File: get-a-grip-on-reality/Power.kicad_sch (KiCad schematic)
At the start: 12 parts, among them J1 Battery Connector, U1 BQ25170DSGR, U2 TLV76733DRVx

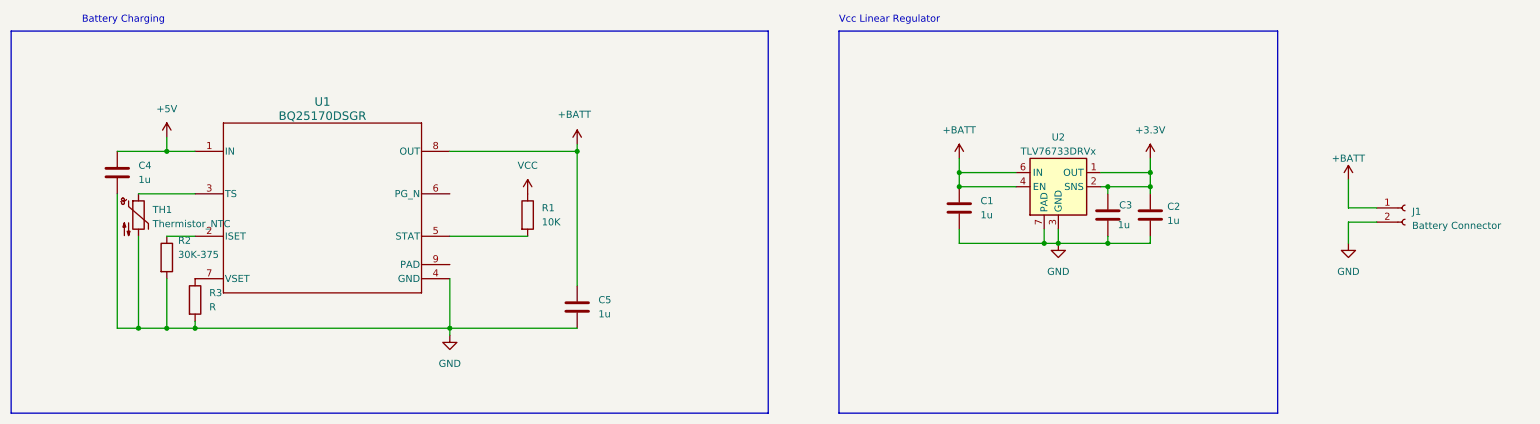
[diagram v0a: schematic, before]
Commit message: power
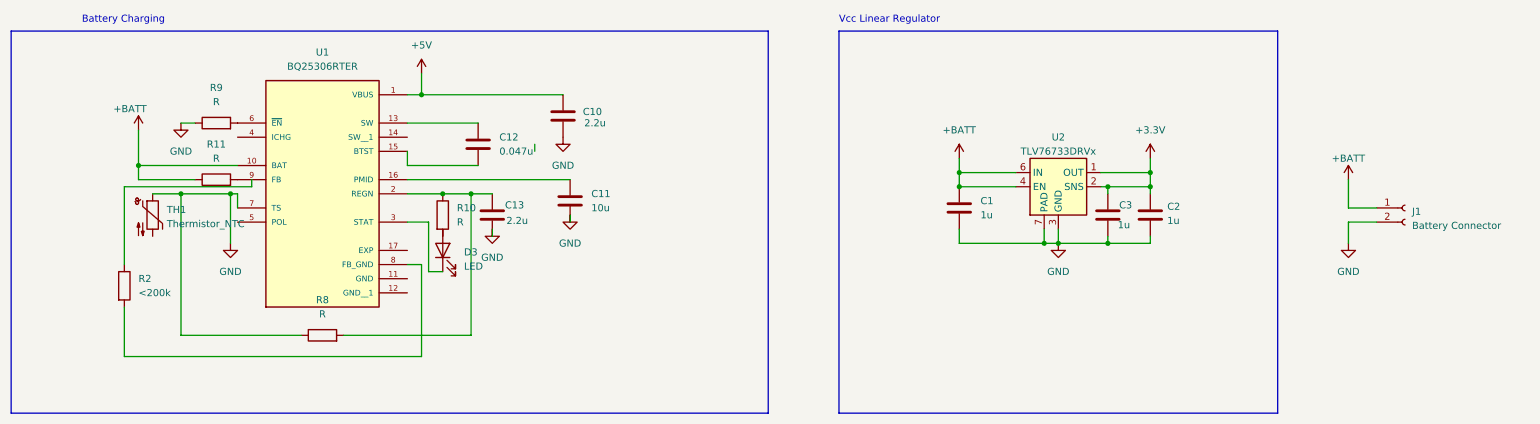
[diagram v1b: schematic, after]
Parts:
- removed C4, C5: 1u, symbol Device:C
- removed R1: 10K, symbol Device:R
- removed R3: R, symbol Device:R
- removed U1: BQ25170DSGR, footprints:DSG0008A, symbol bq25170:BQ25170DSGR
- added C10, C13: 2.2u, symbol Device:C
- added C11: 10u, symbol Device:C
- added C12: 0.047u, symbol Device:C
- added D3: LED, symbol Device:LED
- added R10, R11, R8, R9: R, symbol Device:R
- added U1: BQ25306RTER, BQ25306RTER:IC_BQ25306RTER, symbol BQ25306RTER:BQ25306RTER
- R2: value 30K-375 -> <200k
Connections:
- net +5V: now also C10.1, U1.1 (VBUS)
- net +BATT: now also R11.1, U1.10 (BAT)
- net GND: now also TH1.1, C10.2, C11.2, C13.2, R8.1, R9.1, U1.7 (TS); no longer R2.2, TH1.2
- new net: D3.1 (K), U1.3 (STAT)
- new net: C12.1, U1.13 (SW)
- new net: C12.2, U1.15 (BTST)
- new net: C11.1, U1.16 (PMID)
- new net: C13.1, R10.1, R8.2, U1.2 (REGN)
- new net: R9.2, U1.6 (~{EN})
- new net: R2.2, U1.8 (FB_GND)
- new net: R11.2, U1.9 (FB)
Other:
- moved on the sheet: TH1
